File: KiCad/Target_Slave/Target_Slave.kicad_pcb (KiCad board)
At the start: 2 copper layers, 76.2 x 50.8 mm, 49 parts, among them J1 ICSP, J10 I2C, J2 LED, J3 I2C, J4 I2C, J5 SERVO1, J6 SERVO3, J7 SERVO2, J8 Stepper, J9 I2C, U1 PIC16F1788-IP, U2 TSSP4038

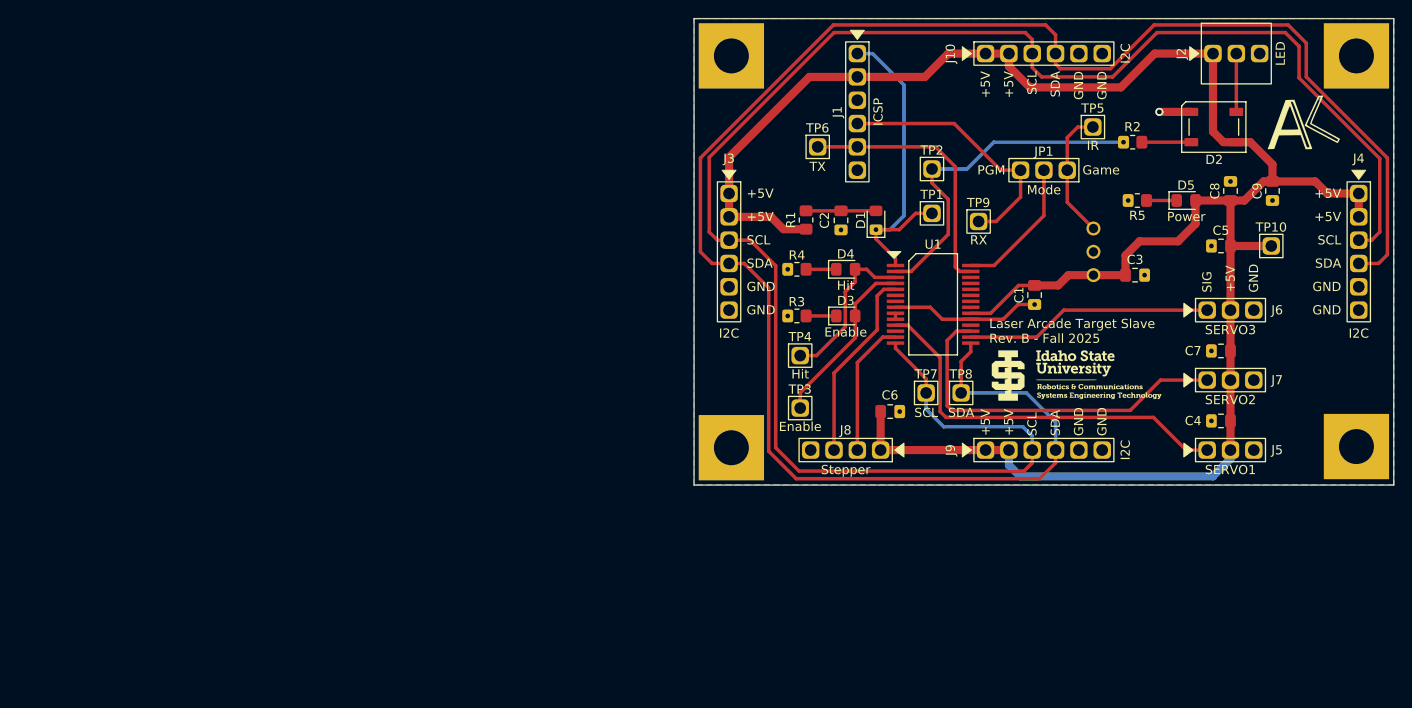
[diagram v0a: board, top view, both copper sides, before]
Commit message: Completed Target Master PCB, export gerbers and views
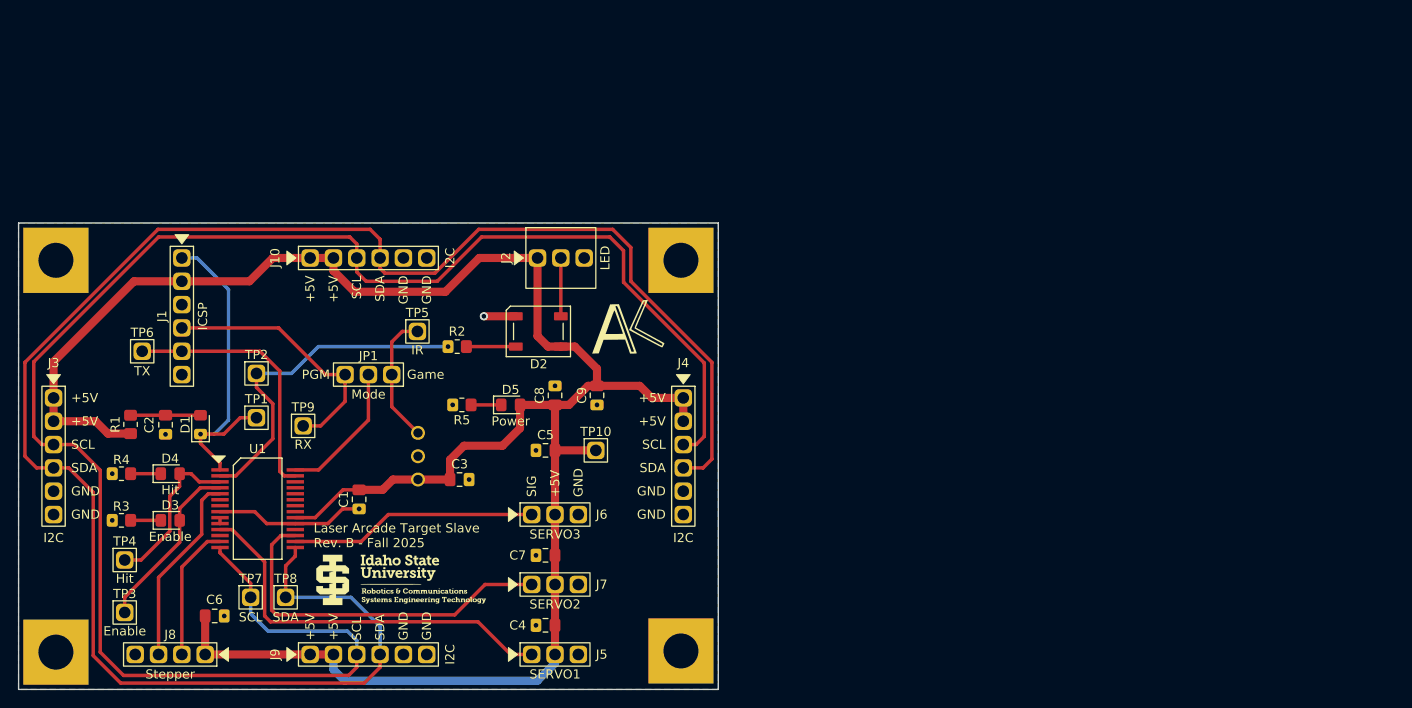
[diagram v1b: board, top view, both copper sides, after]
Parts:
- moved C2 76.9 mm to (119.0, 89.3)
- moved D1 76.9 mm to (122.8, 89.3)
- moved D3 76.9 mm to (119.5, 99.7)
- moved R1 76.9 mm to (115.2, 89.3)
- moved C1 76.9 mm to (140.0, 97.4)
- moved C3 76.9 mm to (151.0, 95.3)
- moved C4 76.9 mm to (160.3, 111.2)
- moved C5 76.9 mm to (160.3, 92.1)
- moved C7 76.9 mm to (160.3, 103.5)
- moved C8 76.9 mm to (161.4, 86.1)
- moved C9 76.9 mm to (166.0, 86.1)
- moved D2 76.9 mm to (159.6, 79.2)
- moved D4 76.9 mm to (119.5, 94.6)
- moved D5 76.9 mm to (156.6, 87.2)
- moved G*** 76.9 mm to (169.4, 78.6)
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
